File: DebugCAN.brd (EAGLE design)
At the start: 65 x 61 mm, 57 parts, among them J1 8P8C-LED, J3 MA04-1, J4 10118192-0001LF, J5 8P8C-LED, J6 8P8C-LED, J7 8P8C-LED, J8 XT60PW-F, U1 STM32F302C, U2 NCV7351D1E, U3 SI8621AB-B-IS, U4 AP2127N-3.3TRG1, U5 78L05F, U6 TLP291, X1 CSTCE8M00G55

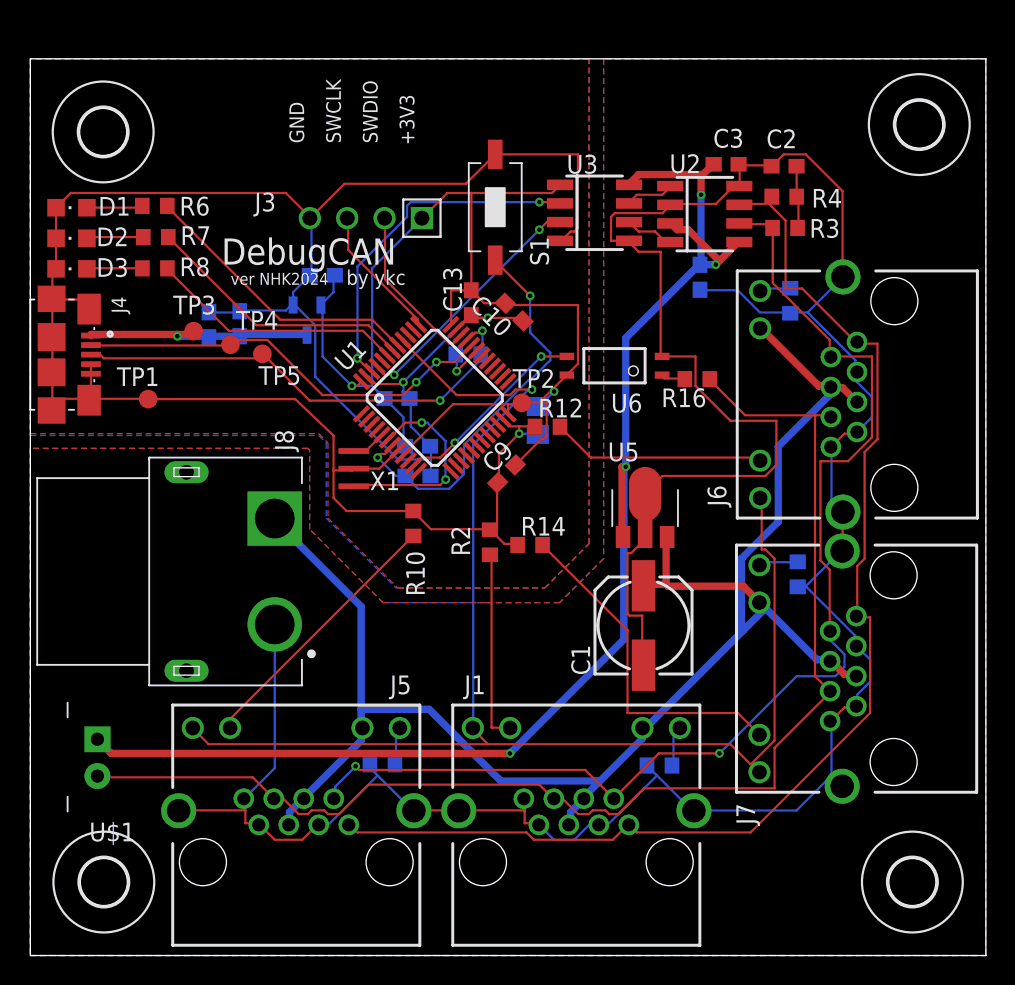
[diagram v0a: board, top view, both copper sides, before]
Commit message: renew position
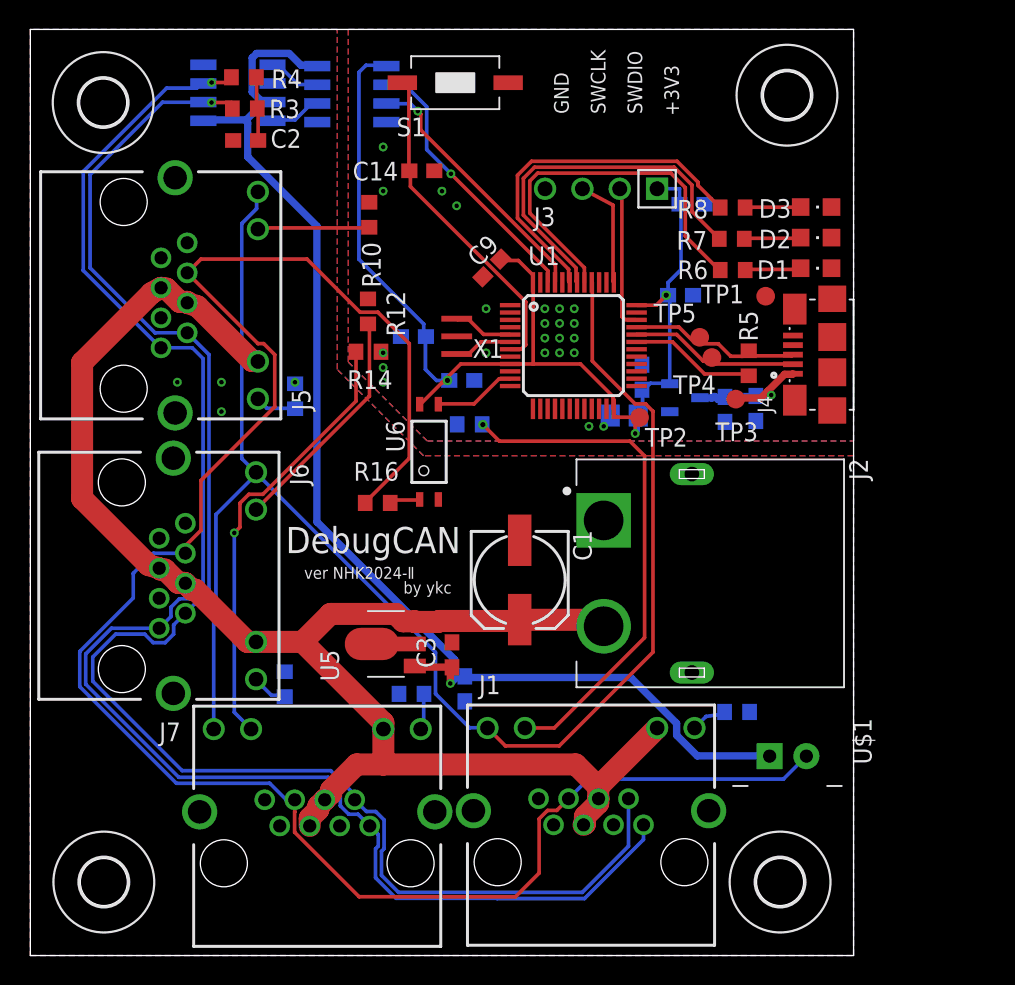
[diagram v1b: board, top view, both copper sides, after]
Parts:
- removed J8: XT60PW-F, con-xt:AMASS_XT60PW-F
- added J2: XT60PW-M, con-xt:AMASS_XT60PW-M
- C3, C4: value (none) -> 100n
- D1: value (none) -> GREEN
- D2: value (none) -> YELLOW
- D3: value (none) -> RED
- R1, R11, R13, R9: value (none) -> 1k
- R10, R12, R14, R2: value (none) -> 470
- moved D3 50.8 mm to (53.5, 50.9), turned to 270 degrees
- moved D1 50.8 mm to (53.5, 46.8), turned to 270 degrees
- moved D2 50.7 mm to (53.5, 48.8), turned to 270 degrees
- moved J4 47.8 mm to (51.9, 40.9), turned to 90 degrees
- moved U$1 47.7 mm to (51.5, 12.8), turned to 180 degrees
- moved R11 43.2 mm to (17.3, 18.5), turned to 270 degrees
- moved TP1 42.6 mm to (50.0, 44.9)
- moved J6 41.7 mm to (12.6, 25.8), turned to 270 degrees
- moved R6 39.6 mm to (47.8, 46.6), turned to 0 degrees
- moved R8 39.5 mm to (47.8, 50.9), turned to 0 degrees
- moved R7 39.2 mm to (47.7, 48.8), turned to 0 degrees
- moved C3 38.2 mm to (28.7, 20.5), turned to 90 degrees
- moved C6 37.6 mm to (49.4, 37.2), turned to 270 degrees
- moved R3 37.6 mm to (14.6, 57.6)
- moved R4 37.6 mm to (14.5, 59.7)
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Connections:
- net +12V: now also J2.2; no longer J8.2
- net GNDIO: now also J2.1; no longer J8.1
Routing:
- net GNDIO: track 198.9 -> 0.00 mm, vias 0 -> 4
- net GNDA: track 171.9 -> 0.00 mm, vias 3 -> 23
- net EMS: track 86.6 -> 130.3 mm
- net CANL: track 80.7 -> 106.9 mm, vias 2 -> 1
- net CANH: track 83.7 -> 107.2 mm, vias 0 -> 1
- net N$4: track 13.1 -> 35.0 mm, vias 0 -> 1
- net USB_DP: track 32.6 -> 12.6 mm, vias 2 -> 0
- net USB_DM: track 29.1 -> 11.8 mm, vias 2 -> 0
- net N$10: track 18.2 -> 7.68 mm
- net N$7: track 14.0 -> 3.97 mm, vias 2 -> 0
- net CAN_LED: track 96.1 -> 104.9 mm, vias 1 -> 0
- net !EMS: track 13.5 -> 5.60 mm, vias 2 -> 0
- net LED2: track 17.5 -> 24.4 mm
- net LED1: track 18.5 -> 25.3 mm
- net N$15: track 23.4 -> 30.1 mm, vias 0 -> 1
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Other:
- board size 65 x 61 mm -> 56 x 63 mm
- board text added: "ver NHK2024-Ⅱ"
- board text removed: "ver NHK2024"
